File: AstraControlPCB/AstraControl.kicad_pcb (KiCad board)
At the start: 4 copper layers, 102 x 96 mm, 150 parts, among them CN1 4P JST VH, CN10 JST_ZH_6PIN_1A_250V, CN2 4P JST VH, CN3 4P JST VH, CN4 4P JST ZH, CN5 4P JST ZH, CN6 4P JST ZH, CN7 JST_VH_8PIN_10A_250V, CN8 4P JST ZH, CN9 4P JST ZH, SW1 TS_Basic_Small, SW2 TS_Basic_Small, U1 ESP32-S3-WROOM-1U-N8, U2 NCP361SNT1G, U3 ST1S12GR, U4 USBLC6-2SC6, U5 THVD2450DGKR, U6 TXB0104PWR

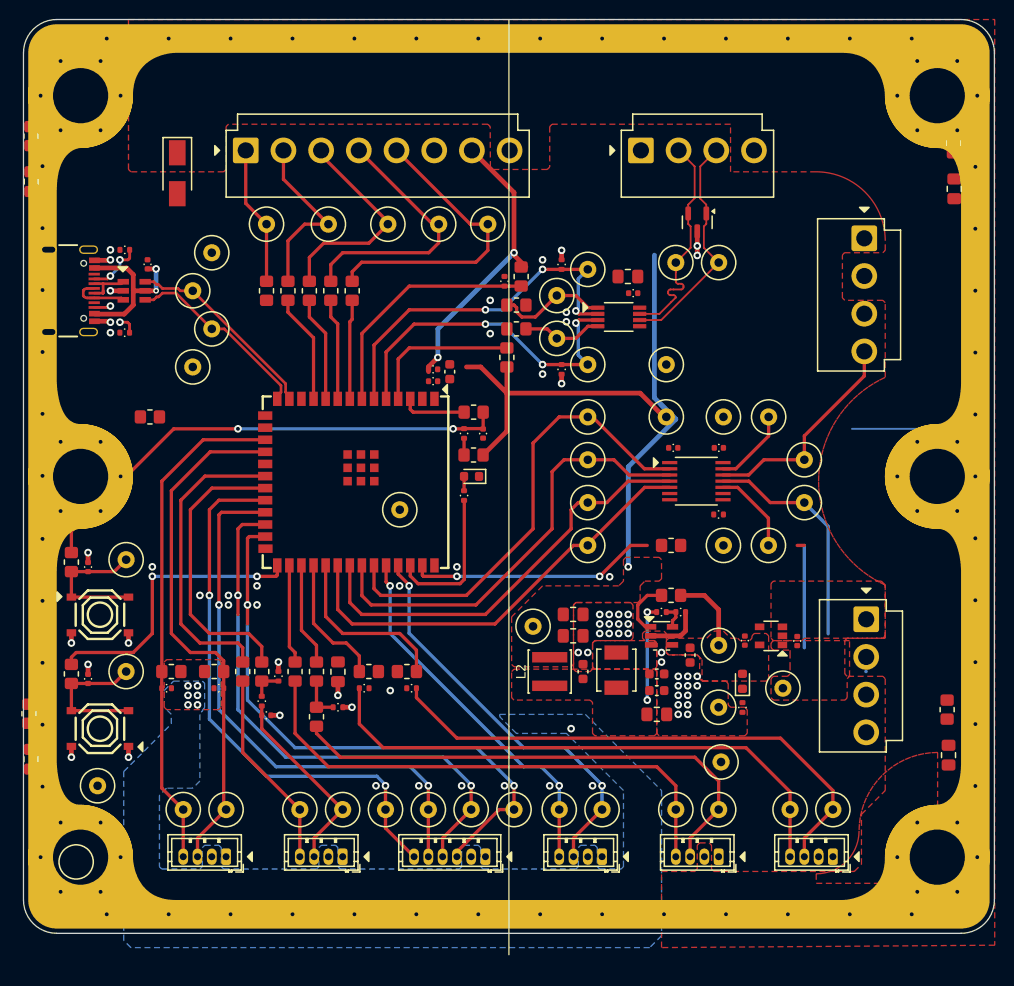
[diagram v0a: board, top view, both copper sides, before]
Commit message: Reroute complete
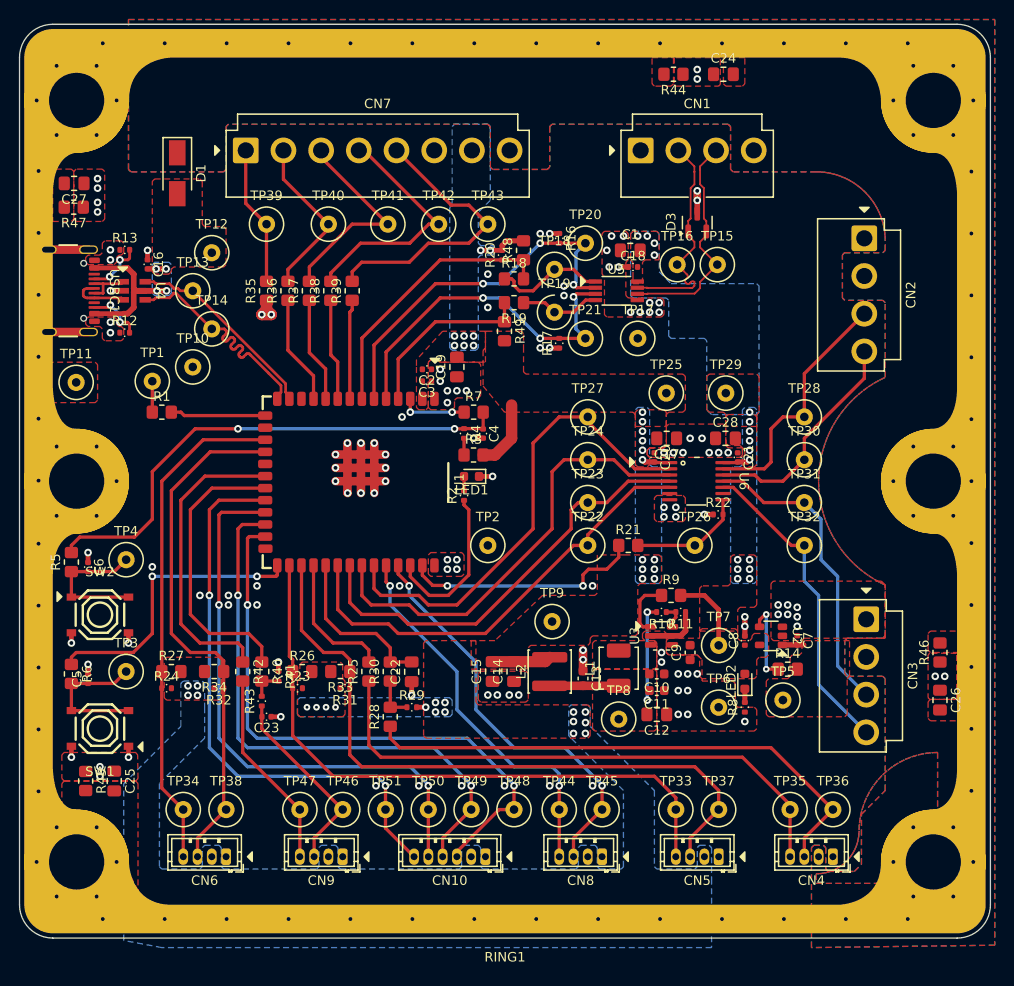
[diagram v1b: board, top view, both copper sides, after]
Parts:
- added C19: 47u, LiveAstra:C_0805_2012Metric_Pad1.18x1.45mm_HandSolder, F.Cu at (144.8, 68.1)
- added C28: DNP, LiveAstra:C_0805_2012Metric_Pad1.18x1.45mm_HandSolder, F.Cu at (173.0, 75.6)
- added R14: 1M, LiveAstra:R_0805_2012Metric_Pad1.20x1.40mm_HandSolder, F.Cu at (179.5, 99.9)
- C1: value 22u -> 47u; footprint LiveAstra:C_0603_1608Metric -> LiveAstra:C_0805_2012Metric_Pad1.18x1.45mm_HandSolder
- moved R45 113.1 mm to (105.8, 111.6), turned to -90 degrees
- moved C25 108.0 mm to (108.8, 111.6), turned to -90 degrees
- moved C24 73.6 mm to (172.8, 37.4), turned to 0 degrees
- moved R44 67.8 mm to (167.5, 37.4), turned to 180 degrees
- moved C27 60.7 mm to (104.6, 48.9), turned to 180 degrees
- moved R47 53.4 mm to (104.5, 51.4), turned to 180 degrees
- moved TP10 53.4 mm to (117.0, 68.1)
- moved TP11 42.4 mm to (104.8, 69.8)
- moved C1 22.9 mm to (163.0, 55.9), turned to 0 degrees
- moved C17 17.5 mm to (166.8, 75.6), turned to 180 degrees
- moved CN4 12.0 mm to (184.3, 119.6)
- moved CN5 12.0 mm to (172.3, 119.6)
- moved TP33 12.0 mm to (167.8, 114.6)
- moved TP35 12.0 mm to (179.8, 114.6)
- moved TP36 12.0 mm to (184.3, 114.6)
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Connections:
- C1 pad 2: +3V3 -> +5V
- C17 pad 2: +5V -> +3V3
- CN1 pad 2: /Block Diagram/UART to RS-485/RS485_IC_D+ -> /Block Diagram/Power Connectors/RS485_D+
- CN1 pad 3: /Block Diagram/UART to RS-485/RS485_IC_D- -> /Block Diagram/Power Connectors/RS485_D-
- D3 pad 1: /Block Diagram/UART to RS-485/RS485_IC_D- -> /Block Diagram/Power Connectors/RS485_D+
- D3 pad 2: /Block Diagram/UART to RS-485/RS485_IC_D+ -> /Block Diagram/Power Connectors/RS485_D-
- TP15 pad 1: /Block Diagram/UART to RS-485/RS485_IC_D- -> /Block Diagram/Power Connectors/RS485_D-
- TP16 pad 1: /Block Diagram/UART to RS-485/RS485_IC_D+ -> /Block Diagram/Power Connectors/RS485_D+
- U1 pad 28: /Block Diagram/Fan, Temperature and Screen/FAN_PWM -> /Block Diagram/Fan, Temperature and Screen/TEMP_I2C_SCL
- U1 pad 29: /Block Diagram/Fan, Temperature and Screen/FAN_TACHO -> /Block Diagram/Fan, Temperature and Screen/TEMP_I2C_SDA
- U1 pad 30: /Block Diagram/Fan, Temperature and Screen/TEMP_I2C_SCL -> /Block Diagram/Fan, Temperature and Screen/FAN_PWM
- U1 pad 31: /Block Diagram/Fan, Temperature and Screen/TEMP_I2C_SDA -> /Block Diagram/Fan, Temperature and Screen/FAN_TACHO
- U2 pad 4: unconnected-(U2-~{FLAG}-Pad4) -> /Block Diagram/5V Protection/FLAG_IC
- U5 pad 6: /Block Diagram/UART to RS-485/RS485_IC_D- -> /Block Diagram/Power Connectors/RS485_D-
- U5 pad 7: /Block Diagram/UART to RS-485/RS485_IC_D+ -> /Block Diagram/Power Connectors/RS485_D+
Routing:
- net +3V3: track 103.4 -> 22.6 mm, vias 12 -> 39
- net GND: track 24.7 -> 65.9 mm, vias 67 -> 125
- net /Block Diagram/UART to RS-485/RS485_IC_D-: track 24.3 -> 0.00 mm
- net /Block Diagram/UART to RS-485/RS485_IC_D+: track 24.2 -> 0.00 mm
- net /Block Diagram/Power Connectors/RS485_D-: track 0.00 -> 24.1 mm
- net /Block Diagram/Power Connectors/RS485_D+: track 0.00 -> 24.0 mm
- net /Block Diagram/3V3 to 5V Logic Shifter/5V_IO_1: track 8.22 -> 26.3 mm
- net /Block Diagram/3V3 to 5V Logic Shifter/5V_IO_4: track 20.5 -> 33.4 mm
- net /Block Diagram/3V3 to 5V Logic Shifter/OE_IC: track 0.00 -> 12.2 mm
- net /Block Diagram/MCU/IO_3_IC: track 0.00 -> 10.0 mm
- net /Block Diagram/5V Protection/FLAG_IC: track 0.00 -> 8.66 mm, vias 0 -> 2
- net CHASSIS: track 0.00 -> 8.37 mm
- net /Block Diagram/3V3 to 5V Logic Shifter/5V_IO_3: track 24.3 -> 32.3 mm
- net /Block Diagram/5V to 3.3V/SW_OUT_UNFILTERED: track 10.2 -> 17.5 mm
- net /Block Diagram/Fan, Temperature and Screen/FAN_TACHO: track 10.8 -> 17.4 mm
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- added copper zone on B.Cu, net +5V
- added copper zone on B.Cu, net +5V_IN
- added copper zone on B.Cu, net /Block Diagram/Power Connectors/USB/VBUS
- added copper zone on F.Cu, net /Block Diagram/Power Connectors/USB/VBUS
- added copper zone on F.Cu, net CHASSIS
